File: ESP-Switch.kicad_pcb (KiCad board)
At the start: 2 copper layers, 119.3 x 58.4 mm, 46 parts, among them K1 Relay, K2 Relay, K3 Relay, K4 Relay, Q1 BC817, Q2 BC817, Q3 BC817, Q4 BC817, U1 AMS1117-3.3

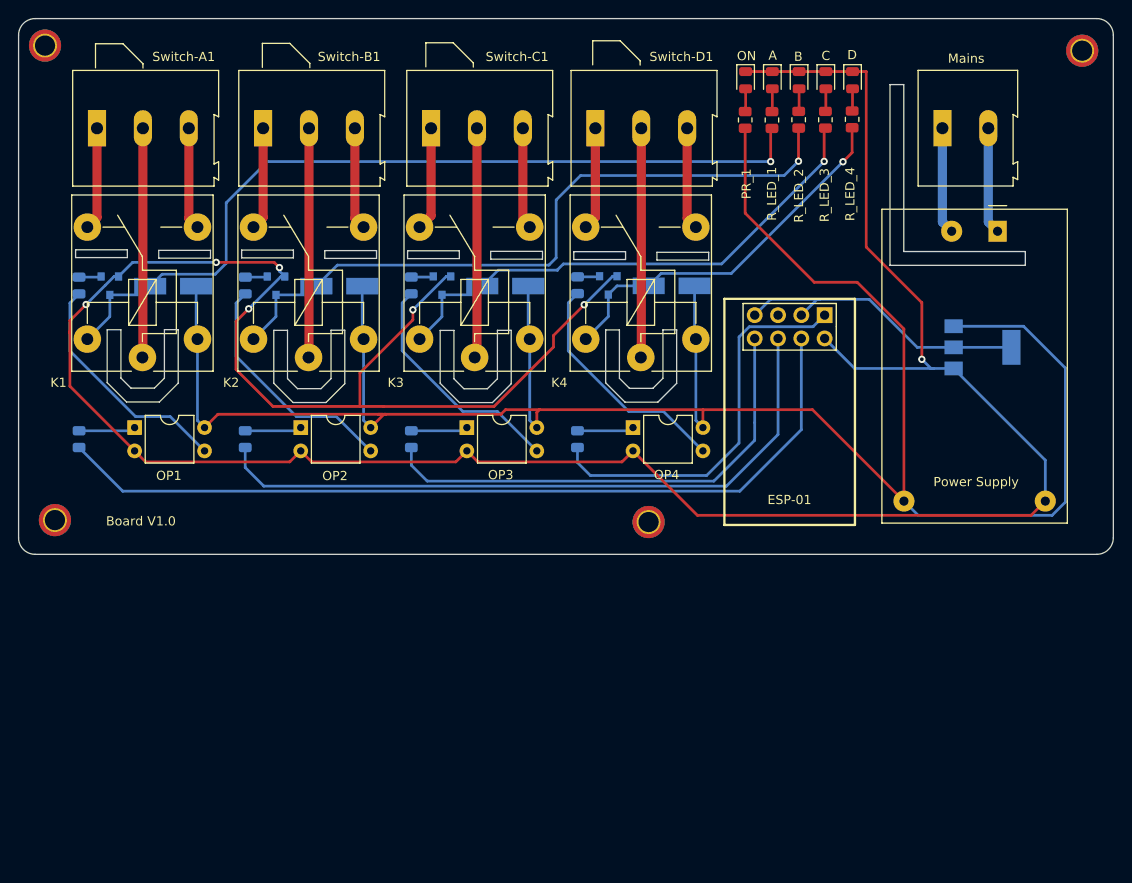
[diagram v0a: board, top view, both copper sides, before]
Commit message: dimmer version
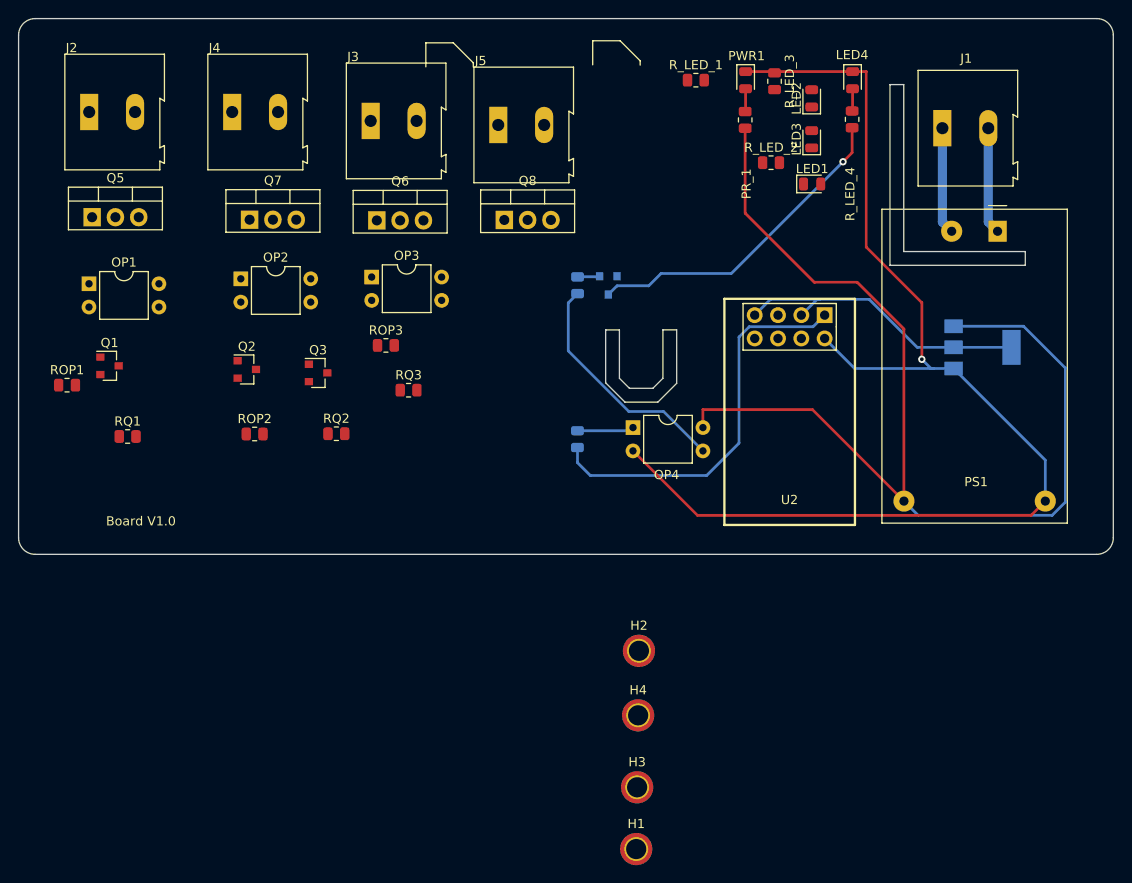
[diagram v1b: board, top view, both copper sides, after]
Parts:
- removed A, B, C: LED, LED_SMD:LED_0805_2012Metric
- removed D1, D2, D3, D4: 1N4007, Diode_SMD:D_SMA_Handsoldering
- removed the H1 at (107.1, 79.1)
- removed the H1 at (154.3, 27.8)
- removed K1, K2, K3, K4: Relay, Relay_THT:Relay_SPDT_Finder_36.11
- removed Switch-A1, Switch-B1, Switch-C1, Switch-D1: Load, TerminalBlock:TerminalBlock_Altech_AK300-3_P5.00mm
- added H1: MountingHole, MountingHole:MountingHole_2.2mm_M2_ISO7380_Pad_TopBottom, F.Cu at (105.8, 114.7)
- added H2: MountingHole, MountingHole:MountingHole_2.2mm_M2_ISO7380_Pad_TopBottom, F.Cu at (106.0, 93.1)
- added J2: Load/Hot, TerminalBlock:TerminalBlock_Altech_AK300-2_P5.00mm, F.Cu at (46.1, 34.4)
- added J3: Load/Hot, TerminalBlock:TerminalBlock_Altech_AK300-2_P5.00mm, F.Cu at (76.8, 35.4)
- added J4: Load/Hot, TerminalBlock:TerminalBlock_Altech_AK300-2_P5.00mm, F.Cu at (61.7, 34.4)
- added J5: Load/Hot, TerminalBlock:TerminalBlock_Altech_AK300-2_P5.00mm, F.Cu at (90.7, 35.9)
- added LED1: LED, LED_SMD:LED_0805_2012Metric, F.Cu at (124.9, 42.3)
- added LED2: LED, LED_SMD:LED_0805_2012Metric, F.Cu at (124.9, 33.0)
- added LED3: LED, LED_SMD:LED_0805_2012Metric, F.Cu at (124.9, 37.4)
- added Q5: BT136-500, Package_TO_SOT_THT:TO-220-3_Vertical, F.Cu at (46.5, 45.9)
- added Q6: BT136-500, Package_TO_SOT_THT:TO-220-3_Vertical, F.Cu at (77.5, 46.2)
- added Q7: BT136-500, Package_TO_SOT_THT:TO-220-3_Vertical, F.Cu at (63.6, 46.2)
- added Q8: BT136-500, Package_TO_SOT_THT:TO-220-3_Vertical, F.Cu at (91.4, 46.2)
- PS1: renamed from Power Supply
- Q1, Q2, Q3: moved to F.Cu
- ROP1, ROP2, ROP3: value 470R -> 1K; moved to F.Cu
- ROP4: value 470R -> 1K
- RQ1, RQ2, RQ3: value 120R -> 1K; moved to F.Cu
- RQ4: value 120R -> 1K
- moved H3 103.4 mm to (105.8, 108.0)
- moved H4 67.0 mm to (106.0, 100.2)
- moved OP3 19.4 mm to (76.9, 52.4)
- moved RQ2 19.0 mm to (73.1, 69.5), turned to 0 degrees
- moved OP2 17.5 mm to (62.7, 52.6)
- moved RQ1 17.3 mm to (50.3, 69.8), turned to 0 degrees
- moved Q3 16.5 mm to (71.1, 62.9), turned to 0 degrees
- moved OP1 16.4 mm to (46.1, 53.1)
- moved RQ3 11.4 mm to (81.0, 64.8), turned to 0 degrees
- moved ROP3 10.6 mm to (78.5, 59.9), turned to 0 degrees
- moved Q2 9.67 mm to (63.3, 62.5), turned to 0 degrees
- moved R_LED_1 9.36 mm to (112.2, 31.0), turned to 0 degrees
- moved Q1 8.73 mm to (48.4, 62.1), turned to 0 degrees
- moved R_LED_3 6.95 mm to (120.8, 31.1), turned to 270 degrees
- moved ROP1 6.02 mm to (43.7, 64.2), turned to 0 degrees
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- renumbered Mains to J1, D to LED4, ON to PWR1, ESP-01 to U2
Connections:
- ROP1 pad 2: Out1 -> Out4
- ROP2 pad 2: Out2 -> Out4
- ROP3 pad 2: Out3 -> Out4
- U2 pad 4: Out1 -> (no net)
- U2 pad 6: Out2 -> (no net)
- U2 pad 8: Out3 -> (no net)
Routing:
- net GND: track 313.6 -> 131.1 mm, vias 7 -> 1
- net +5V: track 249.1 -> 126.0 mm
- net Out1: track 93.4 -> 0.00 mm
- net Net-(Q1-Pad3): track 91.4 -> 0.00 mm, vias 1 -> 0
- net Net-(Q2-Pad3): track 76.1 -> 0.00 mm, vias 1 -> 0
- net Out2: track 73.9 -> 0.00 mm
- net Net-(Q3-Pad3): track 57.2 -> 0.00 mm, vias 1 -> 0
- net Out3: track 53.0 -> 0.00 mm
- net Net-(OP2-Pad3): track 26.2 -> 0.00 mm
- net Net-(OP3-Pad3): track 25.8 -> 0.00 mm
- net Net-(OP1-Pad3): track 25.8 -> 0.00 mm
- net /AC\L3-3: track 25.1 -> 0.00 mm
- net /AC\L1-3: track 25.0 -> 0.00 mm
- net /AC\L4-3: track 25.0 -> 0.00 mm
- net /AC\L2-3: track 25.0 -> 0.00 mm
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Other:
- outline, holes or cut-outs redrawn

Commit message: fixing the problems
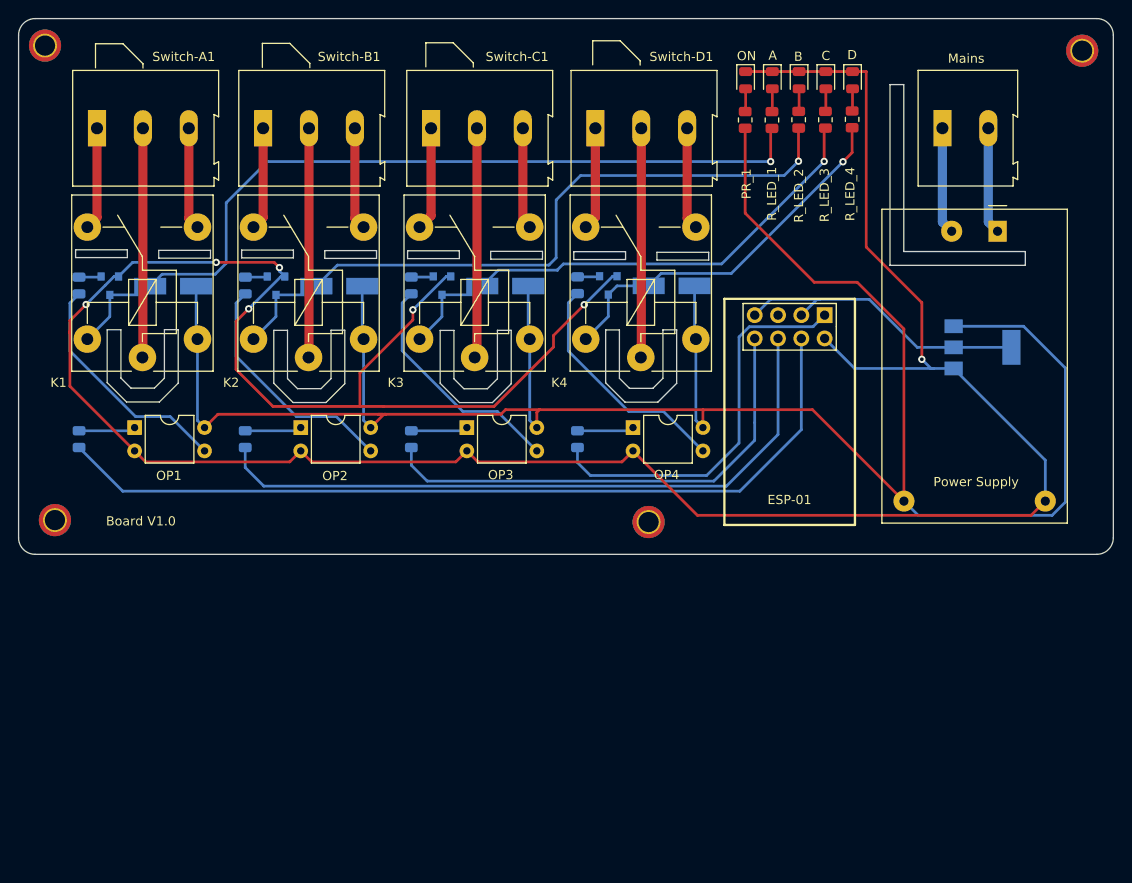
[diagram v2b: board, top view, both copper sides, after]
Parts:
- removed the H1 at (105.8, 114.7)
- removed H2: MountingHole, MountingHole:MountingHole_2.2mm_M2_ISO7380_Pad_TopBottom
- removed J2, J3, J4, J5: Load/Hot, TerminalBlock:TerminalBlock_Altech_AK300-2_P5.00mm
- removed LED1, LED2, LED3: LED, LED_SMD:LED_0805_2012Metric
- removed Q5, Q6, Q7, Q8: BT136-500, Package_TO_SOT_THT:TO-220-3_Vertical
- added A: LED, LED_SMD:LED_0805_2012Metric, F.Cu at (120.6, 31.0)
- added B: LED, LED_SMD:LED_0805_2012Metric, F.Cu at (123.5, 31.0)
- added C: LED, LED_SMD:LED_0805_2012Metric, F.Cu at (126.4, 31.0)
- added D1: 1N4007, Diode_SMD:D_SMA_Handsoldering, B.Cu at (55.3, 53.4)
- added D2: 1N4007, Diode_SMD:D_SMA_Handsoldering, B.Cu at (73.4, 53.4)
- added D3: 1N4007, Diode_SMD:D_SMA_Handsoldering, B.Cu at (91.5, 53.4)
- added D4: 1N4007, Diode_SMD:D_SMA_Handsoldering, B.Cu at (109.6, 53.4)
- added H1: MountingHole, MountingHole:MountingHole_2.2mm_M2_ISO7380_Pad_TopBottom, F.Cu at (107.1, 79.1)
- added H1: MountingHole, MountingHole:MountingHole_2.2mm_M2_ISO7380_Pad_TopBottom, F.Cu at (154.3, 27.8)
- added K1: Relay, Relay_THT:Relay_SPDT_Finder_36.11, F.Cu at (52.0, 61.2)
- added K2: Relay, Relay_THT:Relay_SPDT_Finder_36.11, F.Cu at (70.0, 61.2)
- added K3: Relay, Relay_THT:Relay_SPDT_Finder_36.11, F.Cu at (88.2, 61.2)
- added K4: Relay, Relay_THT:Relay_SPDT_Finder_36.11, F.Cu at (106.2, 61.2)
- added Switch-A1: Load, TerminalBlock:TerminalBlock_Altech_AK300-3_P5.00mm, F.Cu at (47.0, 36.2)
- added Switch-B1: Load, TerminalBlock:TerminalBlock_Altech_AK300-3_P5.00mm, F.Cu at (65.1, 36.2)
- added Switch-C1: Load, TerminalBlock:TerminalBlock_Altech_AK300-3_P5.00mm, F.Cu at (83.4, 36.2)
- added Switch-D1: Load, TerminalBlock:TerminalBlock_Altech_AK300-3_P5.00mm, F.Cu at (101.3, 36.2)
- Power Supply: renamed from PS1
- Q1, Q2, Q3: moved to B.Cu
- ROP1, ROP2, ROP3: value 1K -> 470R; moved to B.Cu
- ROP4: value 1K -> 470R
- RQ1, RQ2, RQ3: value 1K -> 120R; moved to B.Cu
- RQ4: value 1K -> 120R
- moved H3 103.4 mm to (41.3, 27.2)
- moved H4 67.0 mm to (42.4, 78.9)
- moved OP3 19.4 mm to (87.3, 68.8)
- moved RQ2 19.0 mm to (63.2, 53.3), turned to 270 degrees
- moved OP2 17.5 mm to (69.2, 68.8)
- moved RQ1 17.3 mm to (45.0, 53.3), turned to 270 degrees
- moved Q3 16.5 mm to (84.6, 53.4), turned to 270 degrees
- moved OP1 16.4 mm to (51.1, 68.8)
- moved RQ3 11.4 mm to (81.2, 53.3), turned to 270 degrees
- moved ROP3 10.6 mm to (81.2, 70.1), turned to 270 degrees
- moved Q2 9.67 mm to (66.5, 53.4), turned to 270 degrees
- moved R_LED_1 9.36 mm to (120.5, 35.3), turned to 90 degrees
- moved Q1 8.73 mm to (48.4, 53.4), turned to 270 degrees
- moved R_LED_3 6.95 mm to (126.4, 35.3), turned to 90 degrees
- moved ROP1 6.02 mm to (45.0, 70.1), turned to 270 degrees
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- renumbered LED4 to D, U2 to ESP-01, J1 to Mains, PWR1 to ON
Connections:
- ESP-01 pad 4: (no net) -> Out1
- ESP-01 pad 6: (no net) -> Out2
- ESP-01 pad 8: (no net) -> Out3
- ROP1 pad 2: Out4 -> Out1
- ROP2 pad 2: Out4 -> Out2
- ROP3 pad 2: Out4 -> Out3
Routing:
- net GND: track 131.1 -> 313.6 mm, vias 1 -> 7
- net +5V: track 126.0 -> 249.1 mm
- net Out1: track 0.00 -> 93.4 mm
- net Net-(D1-Pad2): track 0.00 -> 91.4 mm, vias 0 -> 1
- net Net-(D2-Pad2): track 0.00 -> 76.1 mm, vias 0 -> 1
- net Out2: track 0.00 -> 73.9 mm
- net Net-(D3-Pad2): track 0.00 -> 57.2 mm, vias 0 -> 1
- net Out3: track 0.00 -> 53.0 mm
- net Net-(OP2-Pad3): track 0.00 -> 26.2 mm
- net Net-(OP3-Pad3): track 0.00 -> 25.8 mm
- net Net-(OP1-Pad3): track 0.00 -> 25.8 mm
- net /AC\L3-3: track 0.00 -> 25.1 mm
- net /AC\L1-3: track 0.00 -> 25.0 mm
- net /AC\L4-3: track 0.00 -> 25.0 mm
- net /AC\L2-3: track 0.00 -> 25.0 mm
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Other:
- outline, holes or cut-outs redrawn
